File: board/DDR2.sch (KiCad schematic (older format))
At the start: 1 part

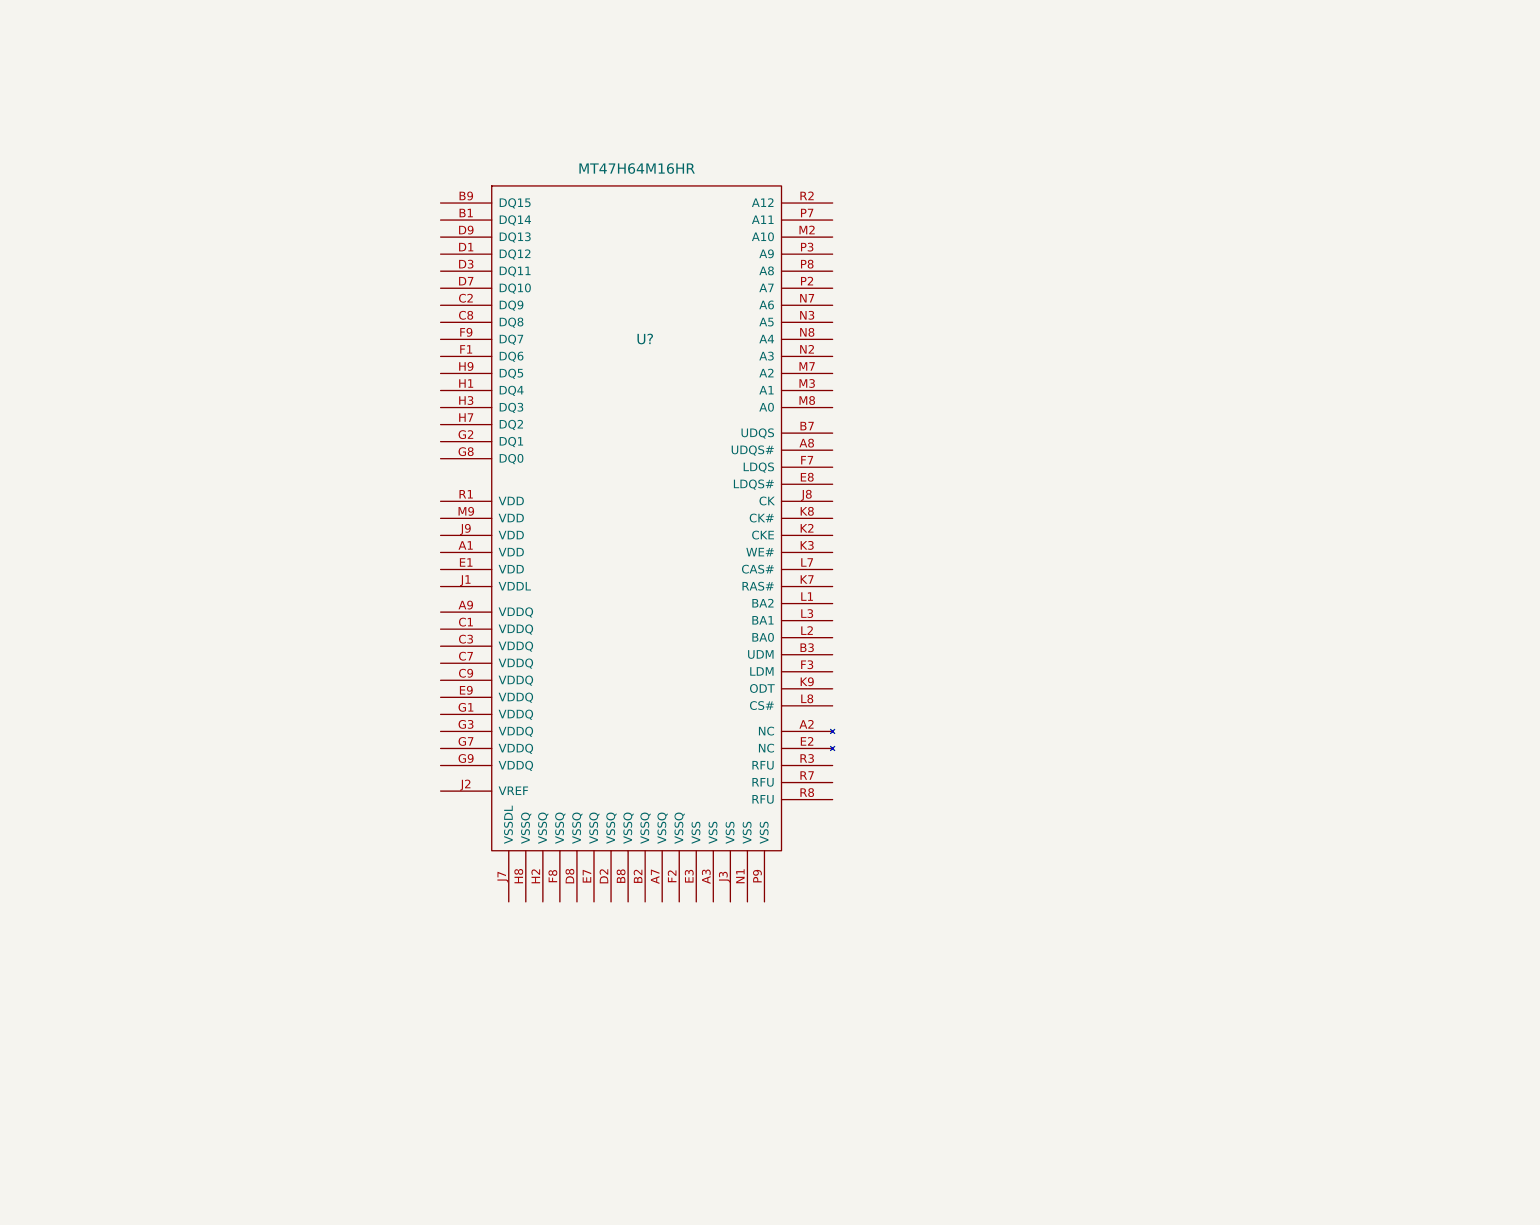
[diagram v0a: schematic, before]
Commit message: Issue #336
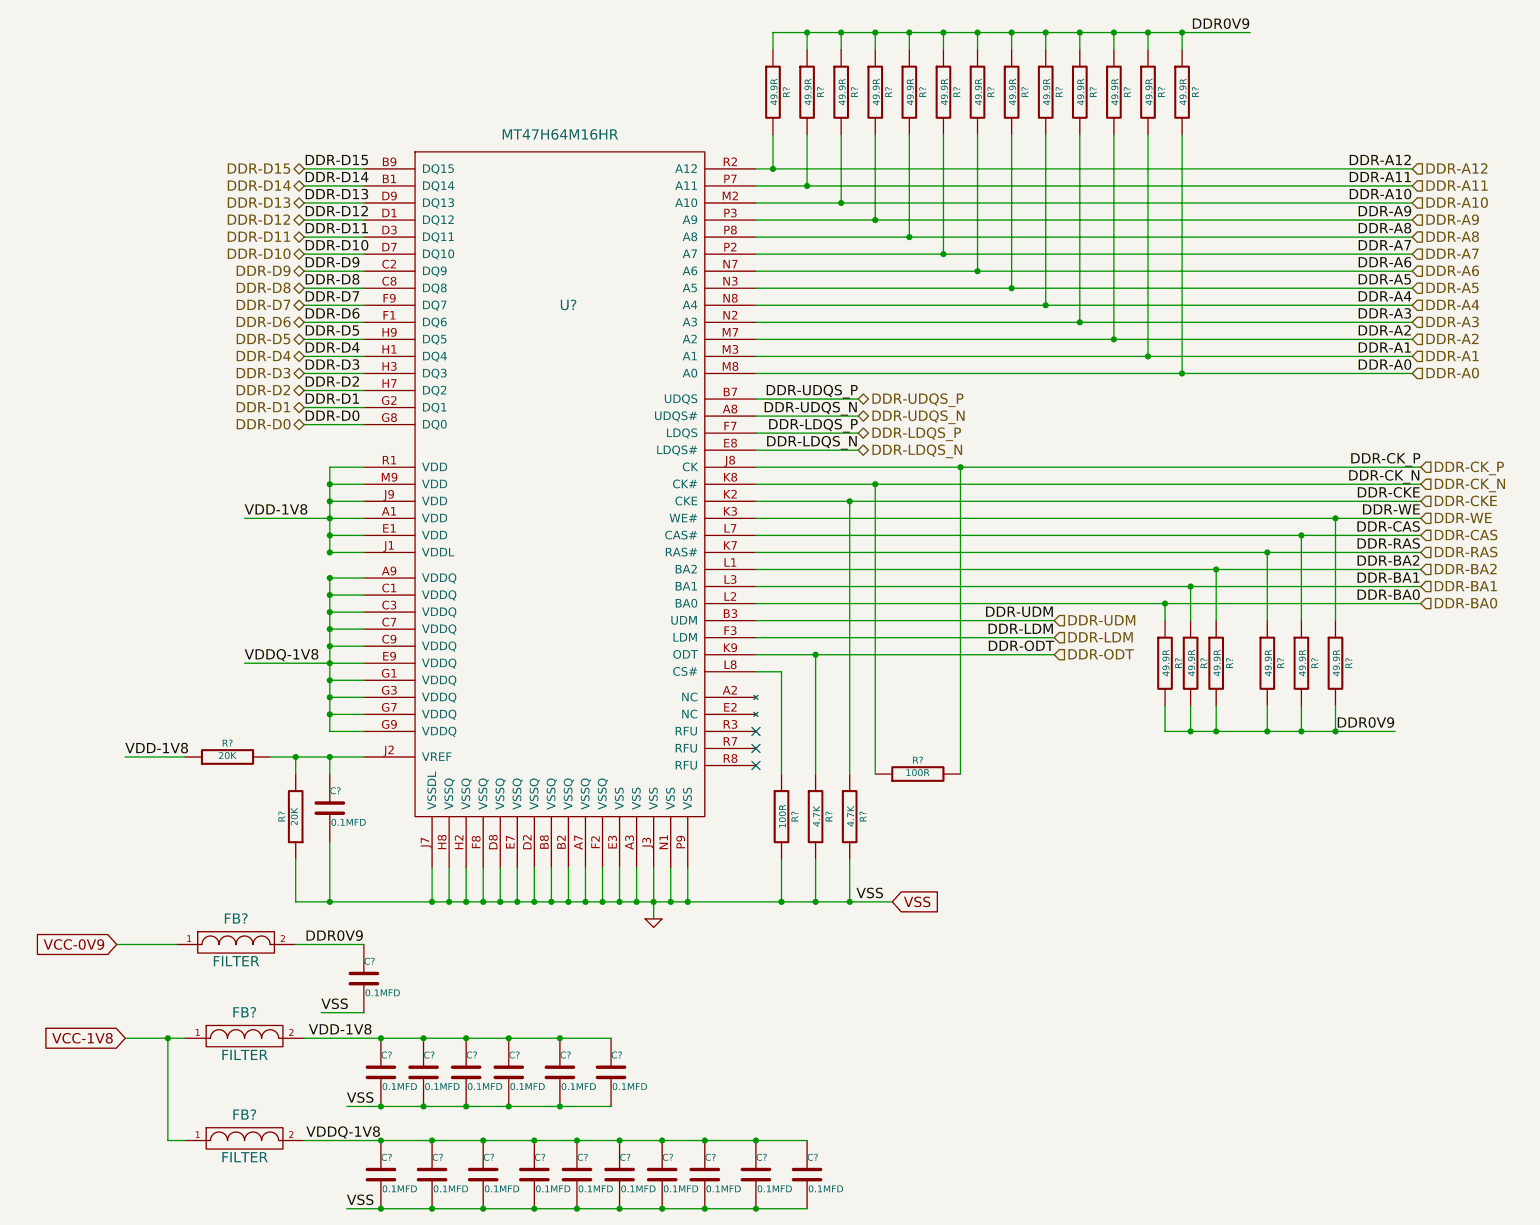
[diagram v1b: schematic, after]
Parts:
- added C? (x18): 0.1MFD, ~, symbol C
- added FB? (x3): FILTER, ~, symbol FILTER
- added R? (x2): 20K, ~, symbol R
- added R? (x19): 49.9R, ~, symbol R
- added R? (x2): 100R, ~, symbol R
- added R? (x2): 4.7K, ~, symbol R
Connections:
- net VDD-1V8: now reaches U?.A1 (VDD)
- net VDD-1V8: now also U?.E1 (VDD), U?.J1 (VDDL), U?.J9 (VDD), U?.M9 (VDD), U?.R1 (VDD), C?.1, C?.1, C?.1, C?.1, C?.1, C?.1, FB?.2, R?.1
- net GND: now reaches U?.A3 (VSS)
- net GND: now also U?.A7 (VSSQ), U?.B2 (VSSQ), U?.B8 (VSSQ), U?.D2 (VSSQ), U?.D8 (VSSQ), U?.E3 (VSS), U?.E7 (VSSQ), U?.F2 (VSSQ), U?.F8 (VSSQ), U?.H2 (VSSQ), U?.H8 (VSSQ), U?.J3 (VSS), U?.J7 (VSSDL), U?.N1 (VSS), U?.P9 (VSS), C?.2, C?.2, C?.2, C?.2, C?.2, C?.2, C?.2, C?.2, C?.2, C?.2, C?.2, C?.2, C?.2, C?.2, C?.2, C?.2, C?.2, C?.2, R?.1, R?.2, R?.2, R?.2
- net DDR-UDQS_N: now reaches U?.A8 (UDQS#)
- net VDDQ-1V8: now reaches U?.A9 (VDDQ)
- net VDDQ-1V8: now also U?.C1 (VDDQ), U?.C3 (VDDQ), U?.C7 (VDDQ), U?.C9 (VDDQ), U?.E9 (VDDQ), U?.G1 (VDDQ), U?.G3 (VDDQ), U?.G7 (VDDQ), U?.G9 (VDDQ), C?.1, C?.1, C?.1, C?.1, C?.1, C?.1, C?.1, C?.1, C?.1, C?.1, FB?.2
- net DDR-D14: now reaches U?.B1 (DQ14)
- net DDR-UDM: now reaches U?.B3 (UDM)
- net DDR-UDQS_P: now reaches U?.B7 (UDQS)
- net DDR-D15: now reaches U?.B9 (DQ15)
- net DDR-D9: now reaches U?.C2 (DQ9)
- net DDR-D8: now reaches U?.C8 (DQ8)
- net DDR-D12: now reaches U?.D1 (DQ12)
- net DDR-D11: now reaches U?.D3 (DQ11)
- net DDR-D10: now reaches U?.D7 (DQ10)
- net DDR-D13: now reaches U?.D9 (DQ13)
- net DDR-LDQS_N: now reaches U?.E8 (LDQS#)
- net DDR-D6: now reaches U?.F1 (DQ6)
- net DDR-LDM: now reaches U?.F3 (LDM)
- net DDR-LDQS_P: now reaches U?.F7 (LDQS)
- net DDR-D7: now reaches U?.F9 (DQ7)
- net DDR-D1: now reaches U?.G2 (DQ1)
- net DDR-D0: now reaches U?.G8 (DQ0)
- net DDR-D4: now reaches U?.H1 (DQ4)
- net DDR-D3: now reaches U?.H3 (DQ3)
- net DDR-D2: now reaches U?.H7 (DQ2)
- net DDR-D5: now reaches U?.H9 (DQ5)
- net at U?.J2 (VREF): now also C?.1, R?.2, R?.2
- net DDR-CK_P: now reaches U?.J8 (CK)
- net DDR-CK_P: now also R?.2
- net DDR-CKE: now reaches U?.K2 (CKE)
- net DDR-CKE: now also R?.1
- net DDR-WE: now reaches U?.K3 (WE#)
- net DDR-WE: now also R?.1
- net DDR-RAS: now reaches U?.K7 (RAS#)
- net DDR-RAS: now also R?.1
- net DDR-CK_N: now reaches U?.K8 (CK#)
- net DDR-CK_N: now also R?.1
- net DDR-ODT: now reaches U?.K9 (ODT)
- net DDR-ODT: now also R?.1
- net DDR-BA2: now reaches U?.L1 (BA2)
- net DDR-BA2: now also R?.1
- net DDR-BA0: now reaches U?.L2 (BA0)
- net DDR-BA0: now also R?.1
- net DDR-BA1: now reaches U?.L3 (BA1)
- net DDR-BA1: now also R?.1
- net DDR-CAS: now reaches U?.L7 (CAS#)
- net DDR-CAS: now also R?.1
- net at U?.L8 (CS#): now also R?.1
- net DDR-A10: now reaches U?.M2 (A10)
- net DDR-A10: now also R?.2
- net DDR-A1: now reaches U?.M3 (A1)
- net DDR-A1: now also R?.2
- net DDR-A2: now reaches U?.M7 (A2)
- net DDR-A2: now also R?.2
- net DDR-A0: now reaches U?.M8 (A0)
- net DDR-A0: now also R?.2
- net DDR-A3: now reaches U?.N2 (A3)
- net DDR-A3: now also R?.2
- net DDR-A5: now reaches U?.N3 (A5)
- net DDR-A5: now also R?.2
- net DDR-A6: now reaches U?.N7 (A6)
- net DDR-A6: now also R?.2
- net DDR-A4: now reaches U?.N8 (A4)
- net DDR-A4: now also R?.2
- net DDR-A7: now reaches U?.P2 (A7)
- net DDR-A7: now also R?.2
- net DDR-A9: now reaches U?.P3 (A9)
- net DDR-A9: now also R?.2
- net DDR-A11: now reaches U?.P7 (A11)
- net DDR-A11: now also R?.2
- net DDR-A8: now reaches U?.P8 (A8)
- net DDR-A8: now also R?.2
- net DDR-A12: now reaches U?.R2 (A12)
- net DDR-A12: now also R?.2
- new net DDR0V9: C?.1, FB?.2, R?.1, R?.1, R?.1, R?.1, R?.1, R?.1, R?.1, R?.1, R?.1, R?.1, R?.1, R?.1, R?.1, R?.2, R?.2, R?.2, R?.2, R?.2, R?.2
- new net VCC-0V9: FB?.1
- new net VCC-1V8: FB?.1, FB?.1
- no-connect marks 0 -> 3
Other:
- moved on the sheet: U?
